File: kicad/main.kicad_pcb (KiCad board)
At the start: 4 copper layers, 24.4 x 18.3 mm, 20 parts, among them J2 LOAD+, J3 LOAD-, J4 BAT+, J5 BAT-, SW1 SW_SPST, U1 ATtiny13-20SS, U2 AO3406

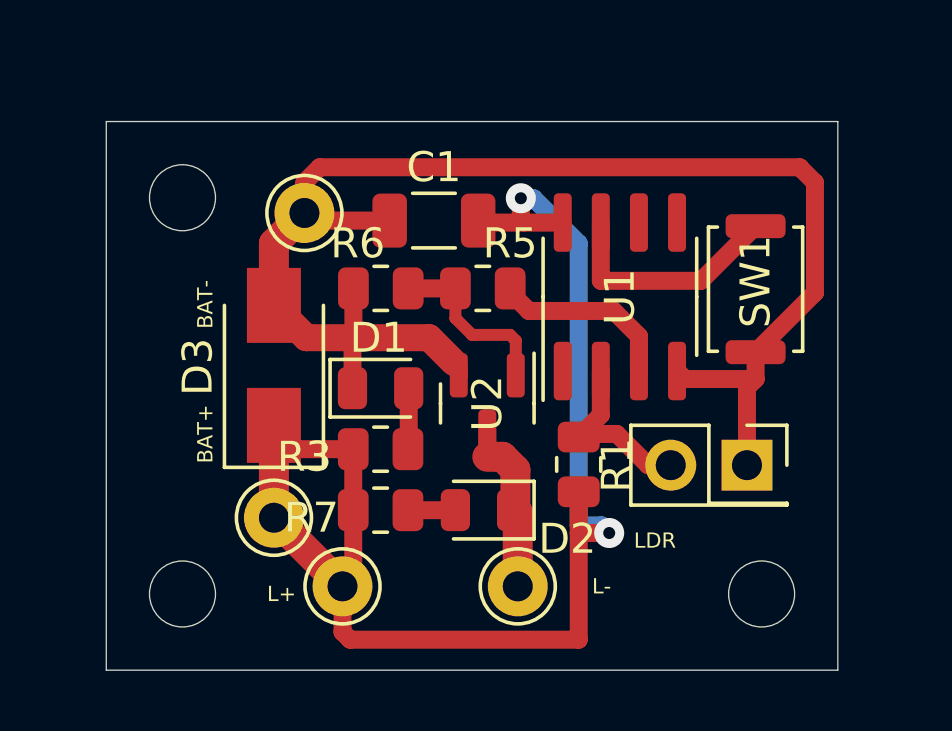
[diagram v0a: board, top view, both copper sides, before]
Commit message: clean up
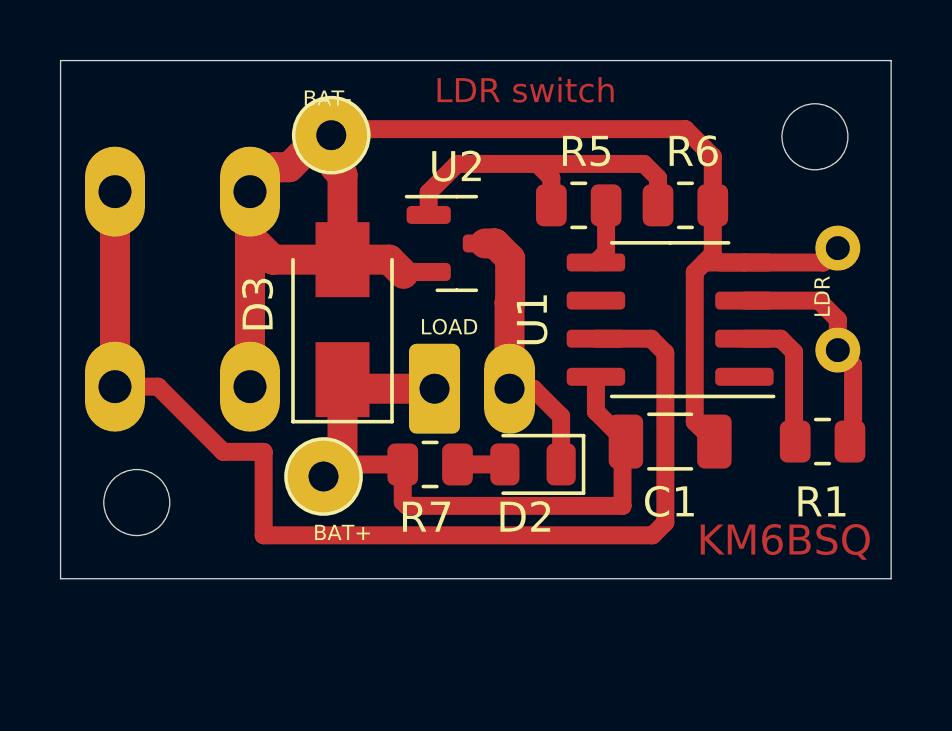
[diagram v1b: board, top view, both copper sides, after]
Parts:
- removed D1: RED, LED_SMD:LED_0805_2012Metric
- removed H2: MountingHole, MountingHole:MountingHole_2.2mm_M2
- removed J3: LOAD-, Connector_Pin:Pin_D1.0mm_L10.0mm
- removed R3: 10k, Resistor_SMD:R_0805_2012Metric
- J2: value LOAD+ -> Conn_LOAD; footprint Connector_Pin:Pin_D1.0mm_L10.0mm -> Connector_JST:JST_XH_B2B-XH-A_1x02_P2.50mm_Vertical; moved to B.Cu
- R2: value LDR -> LDR07; footprint Connector_PinSocket_2.54mm:PinSocket_2x01_P2.54mm_Vertical -> OptoDevice:R_LDR_5.1x4.3mm_P3.4mm_Vertical; moved to B.Cu
- SW1: footprint Button_Switch_SMD:SW_Push_SPST_NO_Alps_SKRK -> Button_Switch_THT:SW_PUSH_6mm; moved to B.Cu
- moved SW1 21.6 mm to (121.4, 58.7)
- moved H3 15.3 mm to (144.8, 56.9)
- moved C1 10.8 mm to (140.0, 67.1), turned to 0 degrees
- moved R6 10.5 mm to (140.5, 59.2), turned to 180 degrees
- moved R1 8.16 mm to (145.0, 67.1), turned to 180 degrees
- moved J2 7.27 mm to (132.1, 65.3)
- moved U2 5.43 mm to (132.8, 60.5), turned to 0 degrees
- moved R2 4.89 mm to (145.5, 64.0), turned to 90 degrees
- moved R5 4.23 mm to (136.9, 59.2)
- moved H1 3.41 mm to (122.2, 69.1)
- moved D3 2.75 mm to (129.0, 63.0)
- moved J5 2.74 mm to (128.7, 56.8)
- moved D2 2.24 mm to (135.4, 67.8)
- moved R7 2.24 mm to (132.0, 67.8)
- moved J4 2.15 mm to (128.4, 68.2)
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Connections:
- R1 pad 2: VCC -> ADC_PWR
- R2 pad 1: GND -> V_REF
- R2 pad 2: V_REF -> GND
- R5 pad 2: Net-(R5-Pad2) -> GATE
- U1 pad 2: V_REF -> ADC_PWR
- U1 pad 3: Net-(R5-Pad2) -> V_REF
- U1 pad 5: MOSI -> GATE
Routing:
- net SCK: track 7.85 -> 36.9 mm
- net VCC: track 46.2 -> 22.1 mm, vias 2 -> 0
- net Net-(R5-Pad2): track 6.21 -> 0.00 mm
- net Net-(R5-Pad1): track 6.05 -> 11.5 mm
- net ADC_PWR: track 0.00 -> 4.84 mm
- net Net-(D2-Pad1): track 5.88 -> 9.10 mm
- net Net-(D1-Pad2): track 2.26 -> 0.00 mm
- net GATE: track 0.00 -> 2.05 mm
- net V_REF: track 6.05 -> 7.69 mm
- net GND: track 48.9 -> 47.5 mm
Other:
- board size 24.4 x 18.3 mm -> 27.7 x 17.3 mm
- board text added: "KM6BSQ"
- board text added: "LDR switch"
- board text added: "LOAD"
- board text added: "LOAD+"
- board text added: "LOAD-"
- board text removed: "L+"
- board text removed: "L-"
